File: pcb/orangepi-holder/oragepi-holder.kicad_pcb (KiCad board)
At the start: 2 copper layers, 96.5 x 64.8 mm, 47 parts, among them J1 Conn_01x02_Male, J2 Conn_01x02_Male, J3 Conn_02x05_Odd_Even, J4 Conn_02x05_Odd_Even, J5 Conn_02x05_Odd_Even, J6 Conn_02x05_Odd_Even, J7 Conn_02x02_Odd_Even, Q1 BD227, Q2 BD227, Q3 BSN10A, Q4 BSN10A, SW1 SW_SPST, SW2 SW_Push, SW3 SW_DPDT_x2, U1 orange_pi_zero, U2 DAC5573

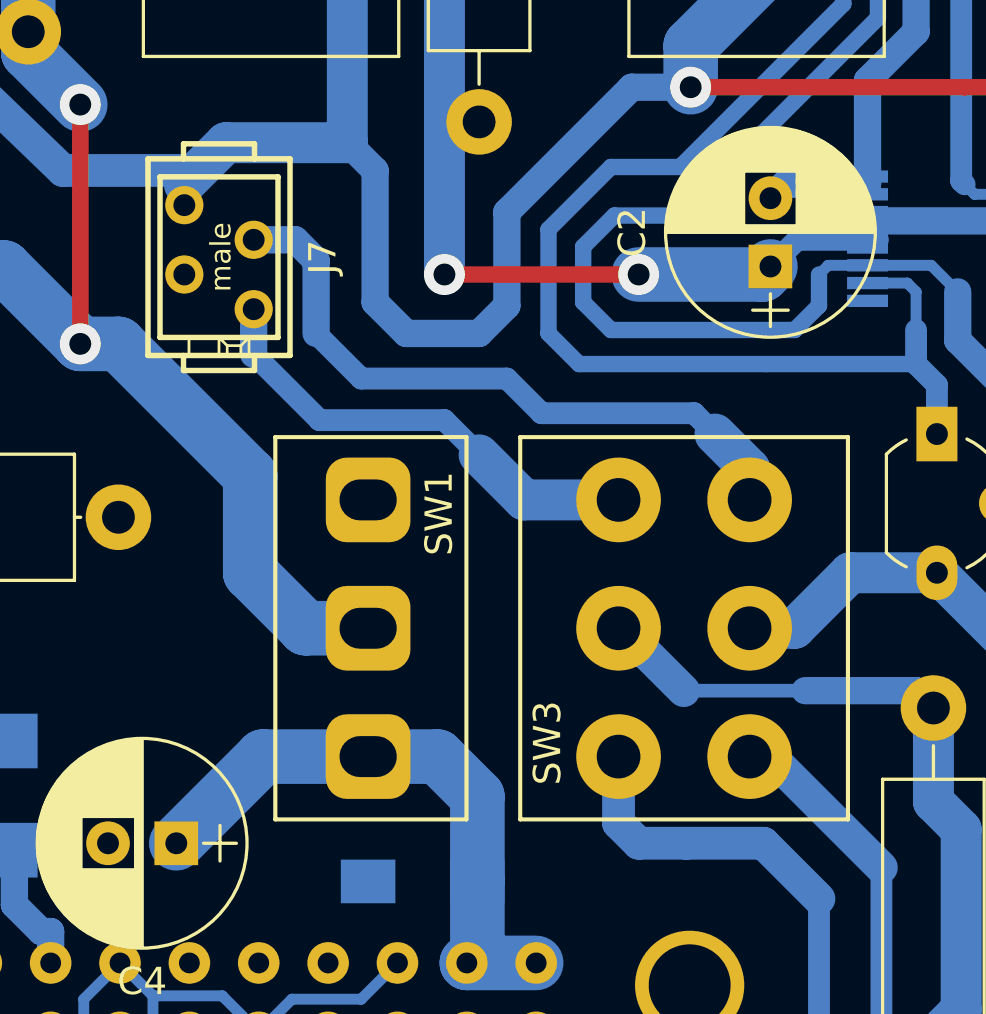
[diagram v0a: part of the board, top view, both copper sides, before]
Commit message: Final orange pi board.
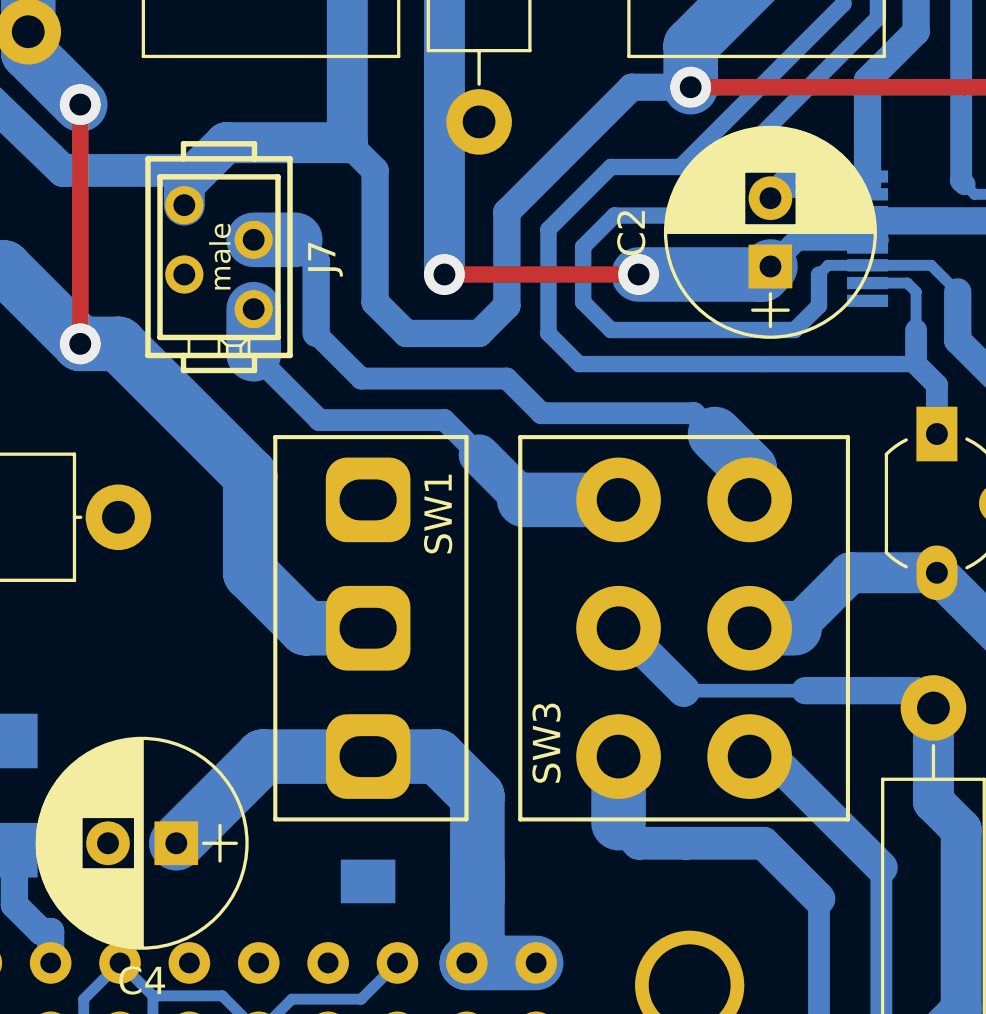
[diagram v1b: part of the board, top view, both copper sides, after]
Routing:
- net +3V3: track 200.0 -> 200.7 mm
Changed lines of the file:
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@@
     (thickness 1.6)
     (drawings 7)
-    (tracks 416)
+    (tracks 417)
     (zones 0)
     (modules 47)
@@
   )
   (setup
-    (last_trace_width 1)
+    (last_trace_width 2)
     (user_trace_width 0.4)
     (user_trace_width 0.5)
@@
   (segment (start 73.025 144.78) (end 68.58 144.78) (width 1.2) (layer B.Cu) (net 6))
   (segment (start 68.58 144.78) (end 65.151 141.478) (width 1.2) (layer B.Cu) (net 6))
+  (segment (start 73.025 146.05) (end 73.025 145.288) (width 1.5) (layer B.Cu) (net 6))
   (segment (start 40.646399 128.898601) (end 40.233599 129.311401) (width 0.4) (layer B.Cu) (net 7))
   (segment (start 40.233599 129.311401) (end 39.37 130.175) (width 0.4) (layer B.Cu) (net 7))
@@
   (segment (start 81.013202 124.968) (end 79.622601 126.358601) (width 1.2) (layer B.Cu) (net 8))
   (segment (start 85.598 124.968) (end 81.013202 124.968) (width 1.2) (layer B.Cu) (net 8))
-  (segment (start 93.726 156.844) (end 93.726 155.702) (width 1.5) (layer B.Cu) (net 9))
-  (segment (start 93.726 155.702) (end 92.456 154.432) (width 1.5) (layer B.Cu) (net 9))
+  (segment (start 93.726 156.844) (end 93.726 155.702) (width 2) (layer B.Cu) (net 9))
+  (segment (start 93.726 155.702) (end 92.456 154.432) (width 2) (layer B.Cu) (net 9))
   (segment (start 92.456 154.432) (end 91.694 153.67) (width 0.8) (layer B.Cu) (net 9))
   (segment (start 91.694 153.67) (end 86.106 153.67) (width 0.8) (layer B.Cu) (net 9))
@@
   (segment (start 79.502 152.4) (end 77.851 150.749) (width 0.8) (layer B.Cu) (net 9))
   (segment (start 77.851 150.749) (end 77.851 148.082) (width 1) (layer B.Cu) (net 9))
-  (segment (start 77.089 147.32) (end 75.565 147.32) (width 1) (layer B.Cu) (net 9))
+  (segment (start 77.089 147.32) (end 75.565 147.32) (width 2) (layer B.Cu) (net 9))
   (segment (start 77.851 148.082) (end 77.089 147.32) (width 1) (layer B.Cu) (net 9))
-  (segment (start 88.926 156.844) (end 85.47 156.844) (width 1.5) (layer B.Cu) (net 10))
+  (segment (start 88.926 156.844) (end 85.47 156.844) (width 2) (layer B.Cu) (net 10))
   (segment (start 85.47 156.844) (end 83.82 155.194) (width 1.5) (layer B.Cu) (net 10))
   (segment (start 83.82 155.194) (end 82.55 153.924) (width 0.8) (layer B.Cu) (net 10))
   (segment (start 82.55 153.924) (end 77.978 153.924) (width 0.8) (layer B.Cu) (net 10))
   (segment (start 77.978 153.924) (end 75.565 151.511) (width 0.8) (layer B.Cu) (net 10))
-  (segment (start 75.565 151.511) (end 75.565 149.86) (width 1) (layer B.Cu) (net 10))
+  (segment (start 75.565 151.511) (end 75.565 149.86) (width 2) (layer B.Cu) (net 10))
   (segment (start 53.909406 170.148) (end 53.877406 170.18) (width 0.8) (layer B.Cu) (net 11))
   (segment (start 54.864 170.148) (end 53.909406 170.148) (width 1) (layer B.Cu) (net 11))
@@
   (segment (start 105.156 164.084) (end 100.584 159.512) (width 1.5) (layer B.Cu) (net 17))
   (segment (start 105.156 164.465) (end 105.156 164.084) (width 1.5) (layer B.Cu) (net 17))
-  (segment (start 93.726 161.544) (end 95.377 161.544) (width 1.5) (layer B.Cu) (net 17))
+  (segment (start 93.726 161.544) (end 95.377 161.544) (width 2) (layer B.Cu) (net 17))
   (segment (start 97.409 159.512) (end 100.584 159.512) (width 1.5) (layer B.Cu) (net 17))
   (segment (start 95.377 161.544) (end 97.409 159.512) (width 1.5) (layer B.Cu) (net 17))
@@
   (segment (start 94.234 169.418) (end 96.266 171.45) (width 1.2) (layer B.Cu) (net 27))
   (segment (start 91.405969 169.418) (end 89.662 169.418) (width 1.2) (layer B.Cu) (net 27))
-  (segment (start 88.926 168.682) (end 88.926 166.244) (width 1.2) (layer B.Cu) (net 27))
+  (segment (start 88.926 168.682) (end 88.926 166.244) (width 2) (layer B.Cu) (net 27))
   (segment (start 89.662 169.418) (end 88.926 168.682) (width 1.2) (layer B.Cu) (net 27))
   (zone (net 2) (net_name GND) (layer B.Cu) (hatch edge 0.508)
